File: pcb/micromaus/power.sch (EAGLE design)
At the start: 27 parts, among them IC1 AD712R, Q1 BSL307SP, T1 BC847, T2 BC847, U1 LP3965EMP-3.3

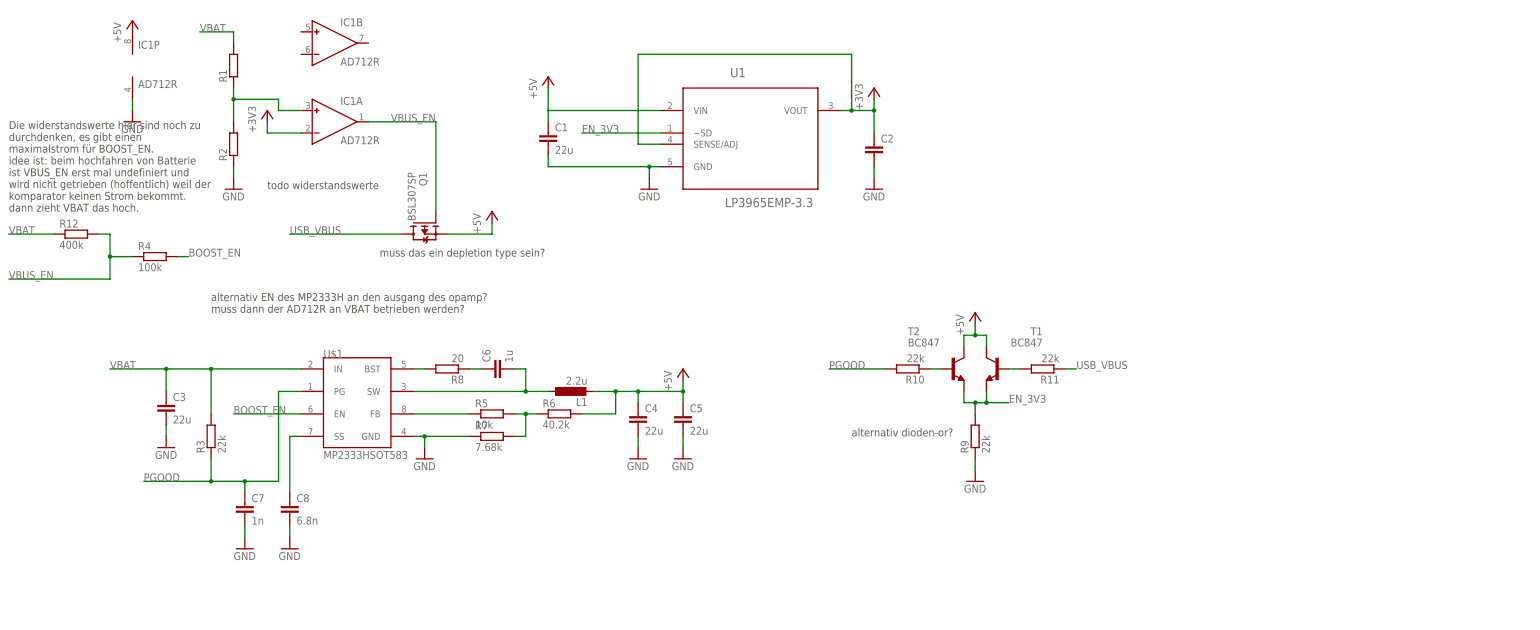
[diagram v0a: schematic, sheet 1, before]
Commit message: improved power supply
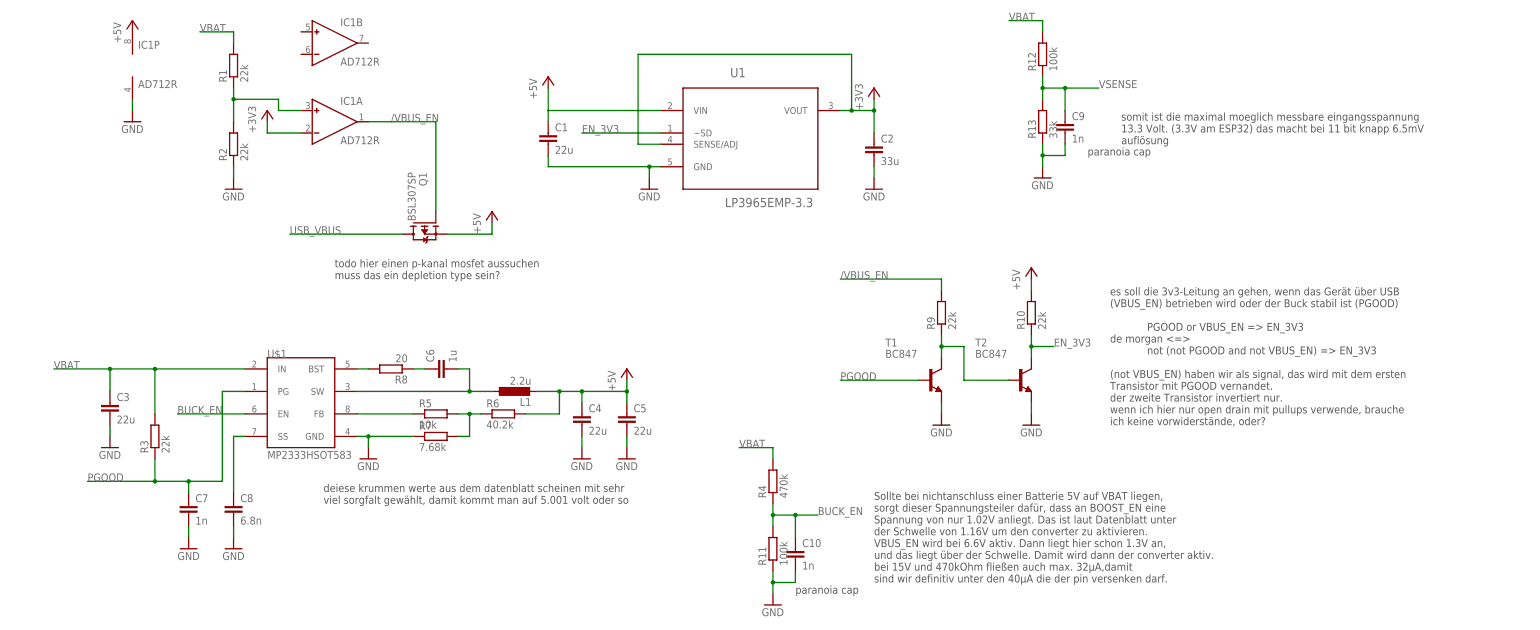
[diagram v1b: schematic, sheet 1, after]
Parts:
- added C10, C9: 1n, rcl:C-EUC0603
- added R13: 33k, rcl:R-EU_R0603
- C2: value (none) -> 33u
- R1, R2: value (none) -> 22k
- R11: value 22k -> 100k
- R12: value 400k -> 100k
- R4: value 100k -> 470k
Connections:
- removed net BOOST_EN: R4.2, U$1.EN
- removed net N$12: R10.1, T2.B
- removed net N$13: R11.2, T1.B
- removed net VBUS_EN: IC1A.OUT, Q1.G, R12.2, R4.1
- new net /VBUS_EN: IC1A.OUT, Q1.G, R9.2
- new net BUCK_EN: C10.1, R11.2, R4.1, U$1.EN
- new net N$1: R9.1, T1.C, T2.B
- new net VSENSE: C9.1, R12.1, R13.2
- net +5V: now also R10.2; no longer T1.C, T2.C
- net EN_3V3: now also R10.1, T2.C; no longer R9.2, T1.E, T2.E
- net GND: now also C10.2, C9.2, R11.1, R13.1, T1.E, T2.E; no longer R9.1
- net PGOOD: now also T1.B; no longer R10.2
- net USB_VBUS: no longer R11.1
- net VBAT: now also R12.2, R4.2; no longer R12.1
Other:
- note added: "Sollte bei nichtanschluss einer Batterie 5V auf VBAT liegen, sorgt dieser Spannungsteiler dafür, dass an BOOST_EN eine Spannung von nur 1.02V anliegt. Das ist laut Datenblatt unter der Schwelle von 1.16V um den converter zu aktivieren. VBUS_EN wird bei 6.6V aktiv. Dann liegt hier schon 1.3V an, und das liegt über der Schwelle. Damit wird dann der converter aktiv. bei 15V und 470kOhm fließen auch 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"
- note added: "deiese krummen werte aus dem datenblatt scheinen mit sehr viel sorgfalt gewählt, damit kommt man auf 5.001 volt oder so"
- note added: "es soll die 3v3-Leitung an gehen, wenn das Gerät über USB (VBUS_EN) betrieben wird oder der Buck stabil ist (PGOOD) PGOOD or VBUS_EN => EN_3V3 de morgan <=> not (not PGOOD and not VBUS_EN) => EN_3V3 (not VBUS_EN) haben wir als signal, das wird mit dem ersten Transistor mit PGOOD vernandet. der zweite Transistor invertiert nur. wenn ich hier nur open drain mit pullups verwende, brauche ich keine v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"
- note added: "paranoia cap"
- note added: "somit ist die maximal moeglich messbare eingangsspannung 13.3 Volt. (3.3V am ESP32) das macht bei 11 bit knapp 6.5mV auflösung"
- note added: "todo hier einen p-kanal mosfet aussuchen muss das ein depletion type sein?"
- note removed: "Die widerstandswerte hier sind noch zu durchdenken, es gibt einen maximalstrom für BOOST_EN. idee ist: beim hochfahren von Batterie ist VBUS_EN erst mal undefiniert und wird nicht getrieben (hoffentlich) weil der komparator keinen Strom bekommt. dann zieht VBAT das hoch."
- note removed: "alternativ EN des MP2333H an den ausgang des opamp? muss dann der AD712R an VBAT betrieben werden?"
- note removed: "alternativ dioden-or?"
- note removed: "muss das ein depletion type sein?"
- note removed: "todo widerstandswerte"
- moved on the sheet: C3, C4, C5, C6, C7, C8, L1, R10, R11, R12, R3, R4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
